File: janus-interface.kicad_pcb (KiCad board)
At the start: 2 copper layers, 40 x 65.5 mm, 12 parts, among them J1 Conn_01x08, J2 Conn_01x04, J3 Conn_01x03, J4 Conn_01x06, J5 Conn_01x02, U1 PHOTON

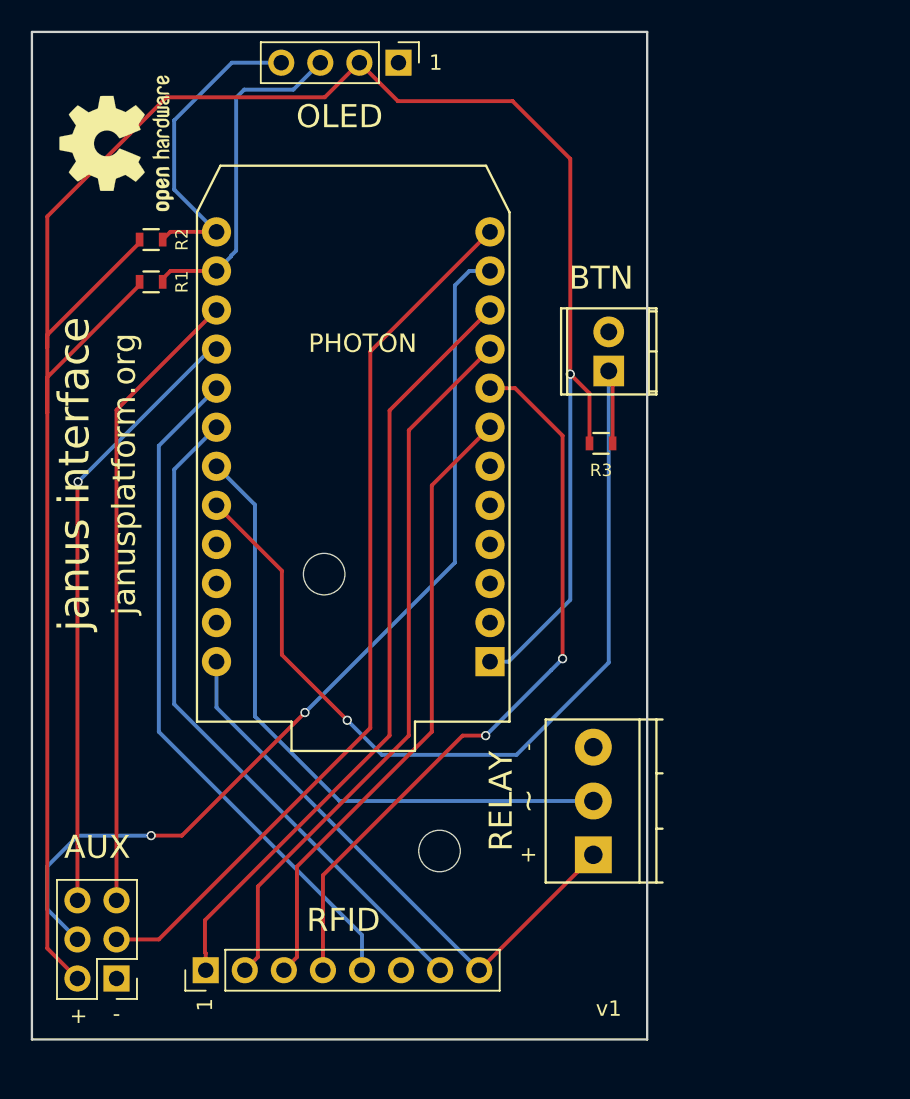
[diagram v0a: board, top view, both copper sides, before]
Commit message: rework board
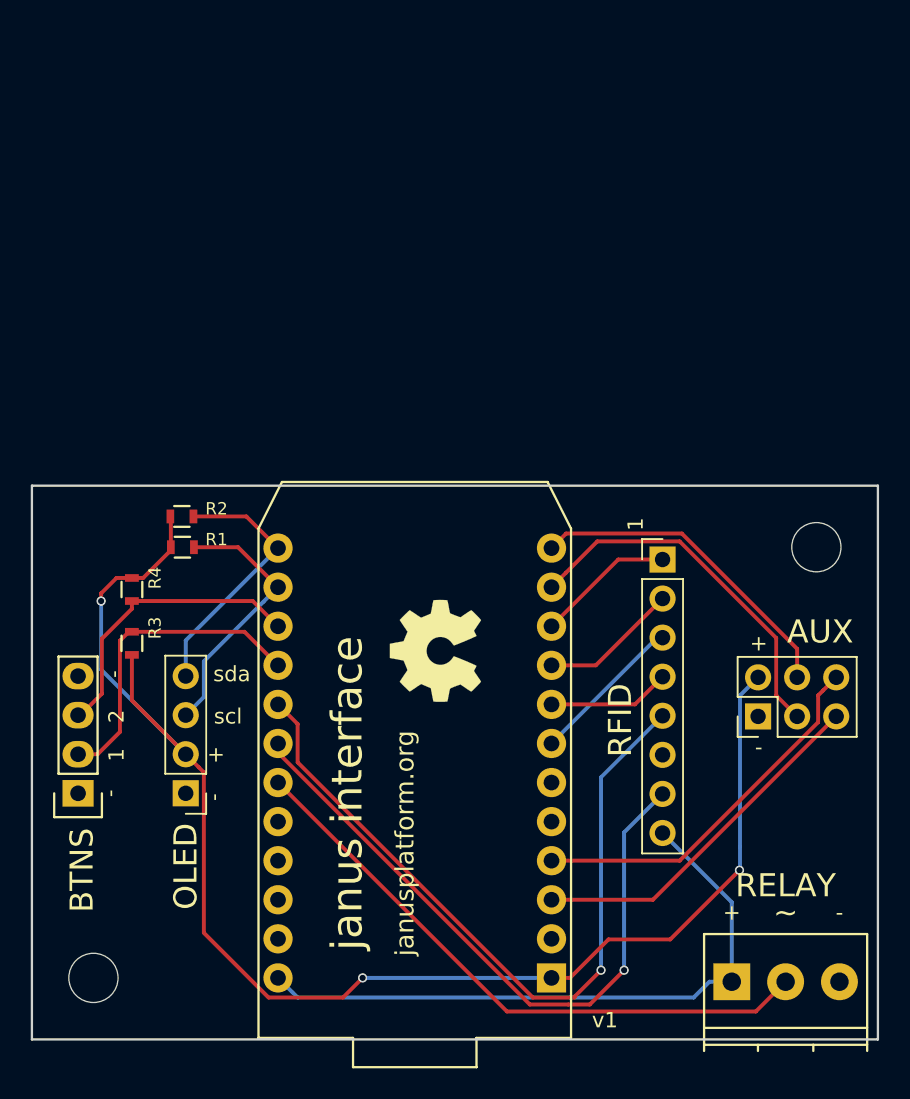
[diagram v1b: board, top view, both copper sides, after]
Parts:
- removed the REF** at (99.0, 129.8)
- removed the REF** at (106.5, 147.8)
- removed the REF*** at (85.5, 101.8)
- added R4: 10k, Resistors_SMD:R_0603, F.Cu at (86.5, 130.8)
- added REF**: MountingHole_3.2mm_M3, Mounting_Holes:MountingHole_3.2mm_M3, F.Cu at (131.0, 128.0)
- added REF**: MountingHole_3.2mm_M3, Mounting_Holes:MountingHole_3.2mm_M3, F.Cu at (84.0, 156.0)
- added REF***: OSHW-Symbol_6.7x6mm_SilkScreen, Symbols:OSHW-Symbol_6.7x6mm_SilkScreen, F.Cu at (106.2, 134.8)
- J5: value Conn_01x02 -> Conn_01x04; footprint Connectors_Terminal_Blocks:TerminalBlock_Pheonix_MPT-2.54mm_2pol -> Pin_Headers:Pin_Header_Straight_1x04
- moved J2 49.5 mm to (90.0, 144.0), turned to 180 degrees
- moved J4 45.1 mm to (127.2, 139.0), turned to 90 degrees
- moved J5 44.1 mm to (83.0, 144.0), turned to 180 degrees
- moved J1 39.9 mm to (121.0, 128.8), turned to 0 degrees
- moved R3 33.2 mm to (86.5, 134.2), turned to 90 degrees
- moved U1 20.9 mm to (104.9, 142.0)
- moved R2 18.1 mm to (89.8, 126.0)
- moved R1 17.4 mm to (89.8, 128.0)
- moved J3 12.2 mm to (125.5, 156.2), turned to 0 degrees
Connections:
- J4 pad 3: /AUX_A0 -> /AUX_A1
- J4 pad 4: /AUX_A1 -> /AUX_A0
- J4 pad 5: /AUX_D2 -> /AUX_TX
- J4 pad 6: /AUX_D3 -> /AUX_RX
- J5 pad 1: /BTN -> /GND
- J5 pad 2: /GND -> /BTN1
- R3 pad 2: /BTN -> /BTN1
- U1 pad 15: /AUX_D2 -> /BTN2
- U1 pad 16: /AUX_D3 -> /BTN1
- U1 pad 20: /BTN -> (no net)
- U1 pad 3: (no net) -> /AUX_TX
- U1 pad 4: (no net) -> /AUX_RX
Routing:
- net /BTN: track 61.7 -> 0.00 mm, vias 1 -> 0
- net /VCC: track 152.1 -> 93.7 mm, vias 1 -> 3
- net /RFID_SS: track 50.6 -> 9.02 mm
- net /AUX_D2: track 41.1 -> 0.00 mm
- net /MISO: track 48.1 -> 7.97 mm, vias 2 -> 0
- net /AUX_D3: track 39.8 -> 0.00 mm, vias 1 -> 0
- net /SCK: track 47.0 -> 9.02 mm
- net /AUX_A1: track 60.9 -> 24.1 mm, vias 2 -> 0
- net /AUX_A0: track 57.7 -> 21.3 mm
- net /MOSI: track 40.9 -> 10.1 mm
- net /AUX_RX: track 0.00 -> 24.5 mm
- net /AUX_TX: track 0.00 -> 23.4 mm
- net /BTN1: track 0.00 -> 20.7 mm
- net /BTN2: track 0.00 -> 19.1 mm
- net /SCL: track 22.1 -> 17.3 mm
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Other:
- board size 40 x 65.5 mm -> 55 x 36 mm
- board text added: "2"
- board text added: "BTNS"
- board text added: "scl"
- board text added: "sda"
- board text removed: "BTN"
